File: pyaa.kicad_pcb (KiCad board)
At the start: 2 copper layers, 123.4 x 80.1 mm, 18 parts, among them J1 MJ-4PP-9, K0 KEYSW, K1 KEYSW, SW1 SW_PUSH, U1 ProMicro

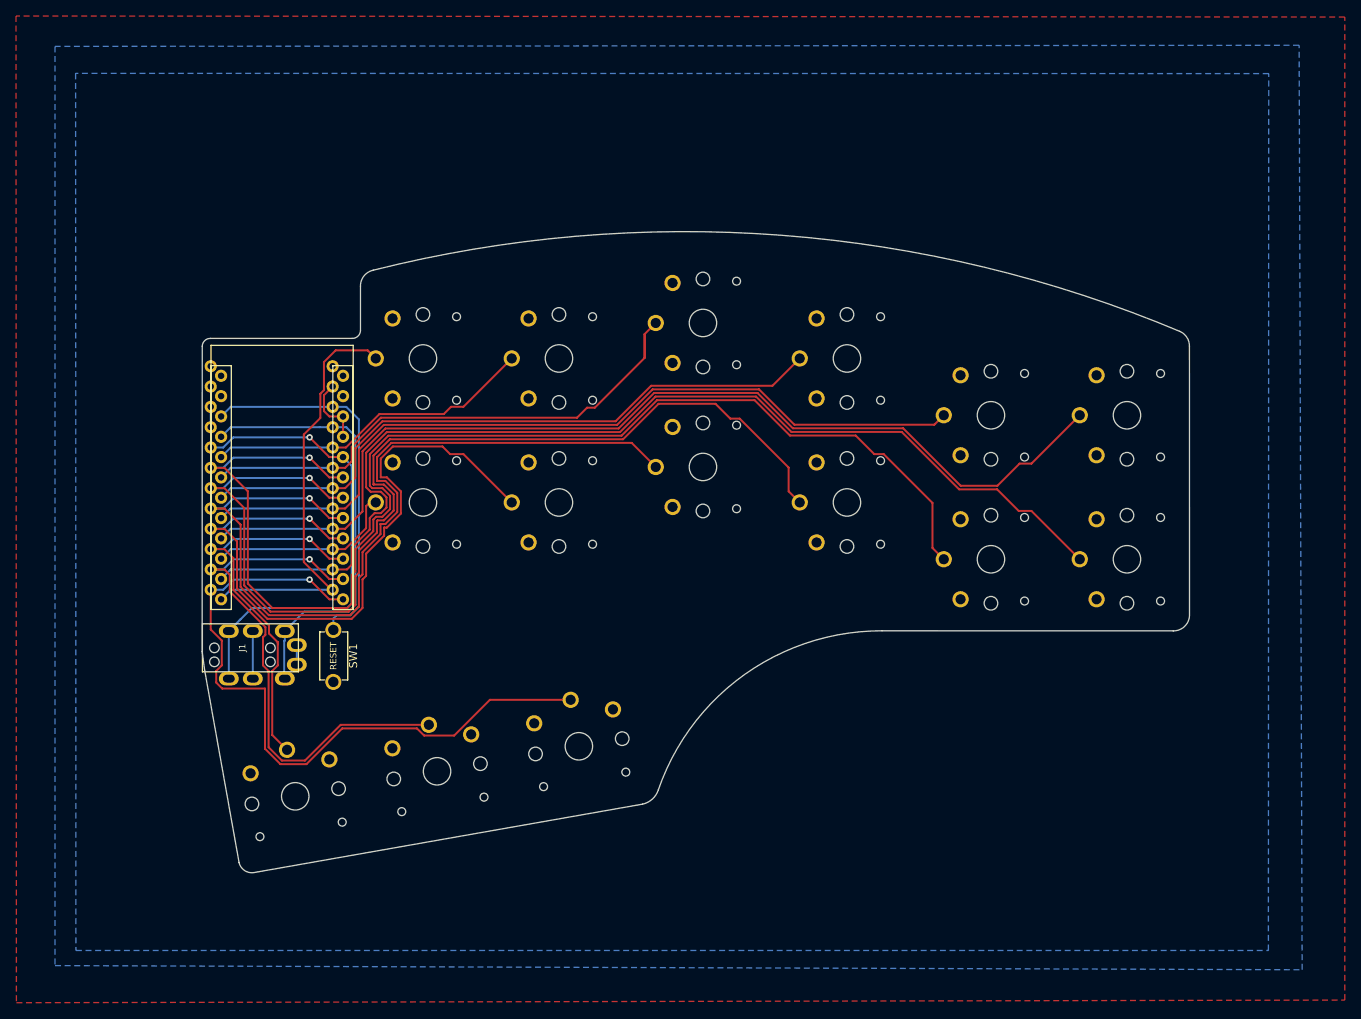
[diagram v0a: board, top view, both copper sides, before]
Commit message: Add files via upload
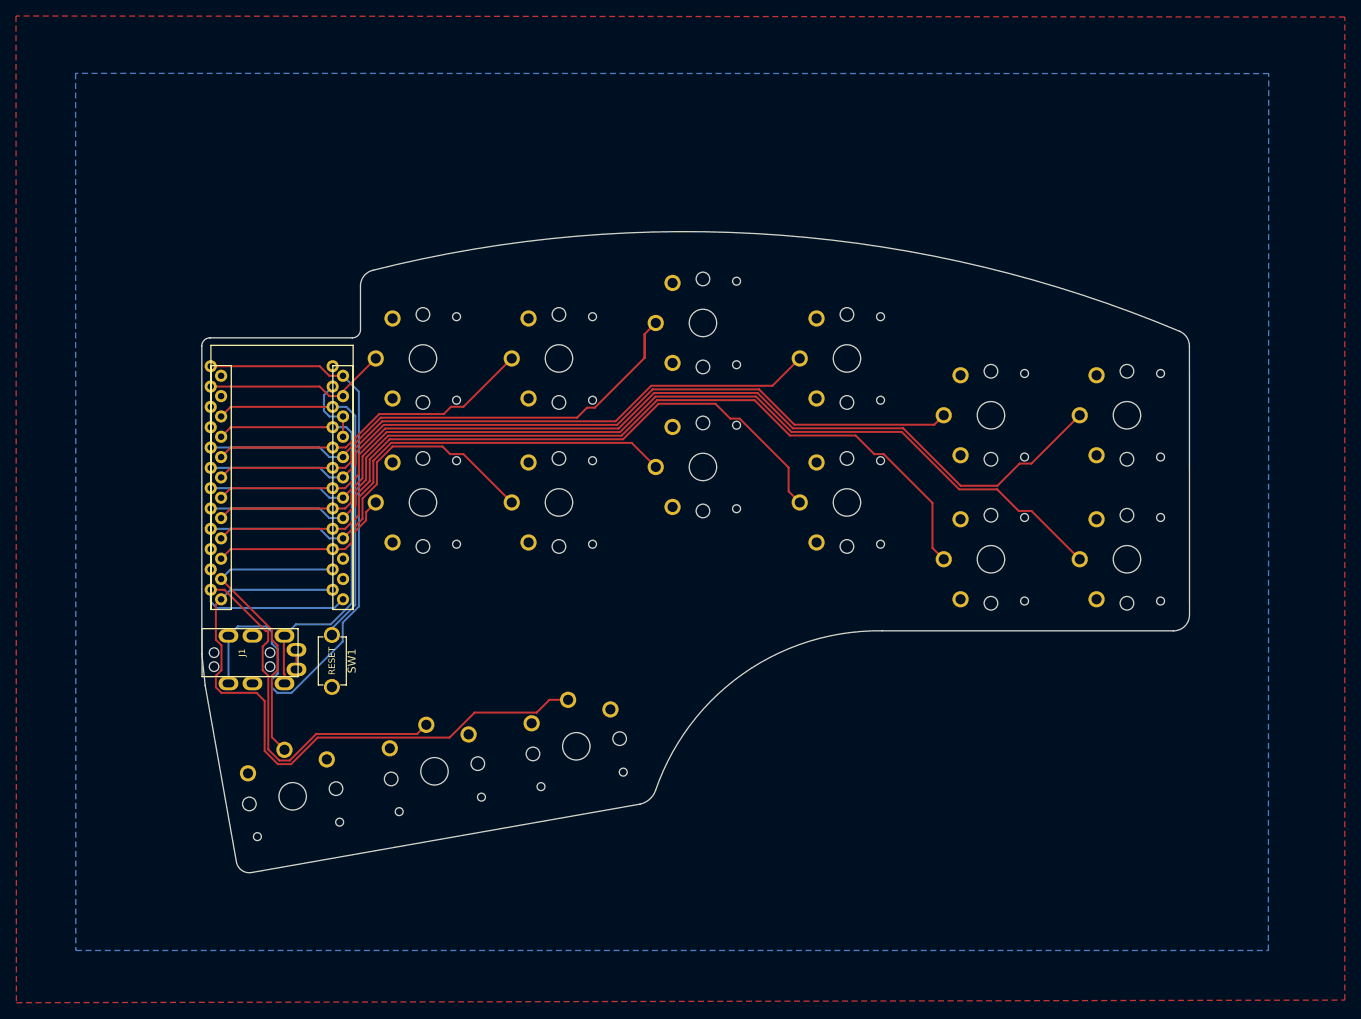
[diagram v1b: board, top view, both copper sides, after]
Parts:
- moved SW1 0.66 mm to (107.9, 113.0)
- moved J1 0.60 mm to (91.6, 112.0)
- moved KA1 0.32 mm to (120.7, 126.8)
- moved KN1 0.32 mm to (138.4, 123.7)
- moved KO1 0.32 mm to (103.0, 129.9)
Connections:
- U1 pad 1: Net-(U1-Pad1) -> Net-(J1-PadB)
- U1 pad 10: Net-(KO1-Pad1) -> Net-(U1-Pad10)
- U1 pad 11: Net-(KA1-Pad1) -> Net-(U1-Pad11)
- U1 pad 12: Net-(KN1-Pad1) -> Net-(KA1-Pad1)
- U1 pad 13: Net-(KST1-Pad1) -> Net-(KN1-Pad1)
- U1 pad 14: Net-(K1-Pad1) -> Net-(KO1-Pad1)
- U1 pad 16: Net-(K0-Pad1) -> Net-(KWL1-Pad1)
- U1 pad 17: Net-(KS1-Pad1) -> Net-(KS2-Pad1)
- U1 pad 18: Net-(KTL1-Pad1) -> Net-(K0-Pad1)
- U1 pad 19: Net-(KPL1-Pad1) -> Net-(KTL1-Pad1)
- U1 pad 2: Net-(U1-Pad2) -> Net-(KST1-Pad1)
- U1 pad 5: Net-(J1-PadB) -> Net-(KPL1-Pad1)
- U1 pad 6: Net-(KS2-Pad1) -> Net-(KS1-Pad1)
- U1 pad 7: Net-(KKL1-Pad1) -> Net-(K1-Pad1)
- U1 pad 8: Net-(KWL1-Pad1) -> Net-(KKL1-Pad1)
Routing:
- net Net-(KS2-Pad1): track 159.0 -> 110.2 mm, vias 1 -> 0
- net Net-(KKL1-Pad1): track 134.3 -> 89.2 mm, vias 1 -> 0
- net Net-(KWL1-Pad1): track 106.6 -> 63.4 mm, vias 1 -> 0
- net Net-(KRL1-Pad1): track 88.0 -> 48.9 mm, vias 1 -> 0
- net Net-(KST1-Pad1): track 53.0 -> 23.4 mm
- net Net-(J1-PadB): track 59.7 -> 83.4 mm, vias 1 -> 0
- net Net-(K1-Pad1): track 135.7 -> 124.4 mm
- net Net-(KO1-Pad1): track 49.0 -> 39.7 mm, vias 1 -> 0
- net Net-(KN1-Pad1): track 87.6 -> 81.3 mm, vias 1 -> 0
- net GND: track 17.2 -> 11.3 mm
- net Net-(K0-Pad1): track 127.7 -> 122.6 mm
- net Net-(KS1-Pad1): track 102.6 -> 99.9 mm
- net Net-(KTL1-Pad1): track 81.7 -> 79.2 mm
- net Net-(KA1-Pad1): track 67.1 -> 65.7 mm, vias 1 -> 0
- net Net-(SW1-Pad1): track 47.0 -> 46.4 mm
- removed copper zone on B.Cu, net (none)
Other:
- board size 123.4 x 80.1 mm -> 123.5 x 80.1 mm
